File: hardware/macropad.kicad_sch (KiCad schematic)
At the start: 28 parts, among them J1 OLED_128x32, SW1 RotaryEncoder_Switch, U1 Raspberry_Pi_Pico, U2 ESP32-WROOM-32

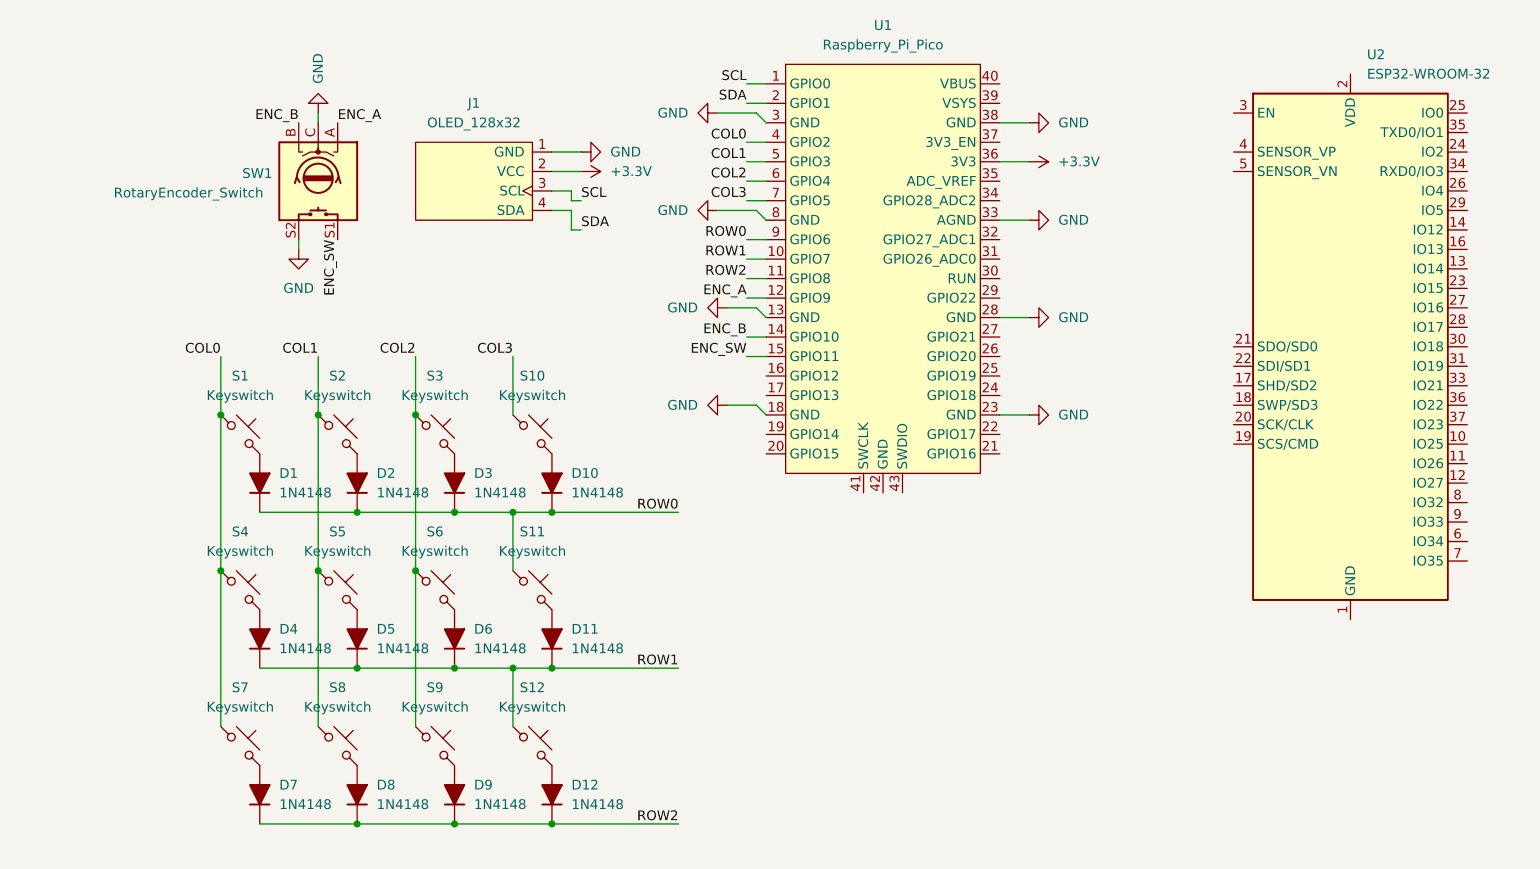
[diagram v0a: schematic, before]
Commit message: updated schematic, removed everything from pcbnew
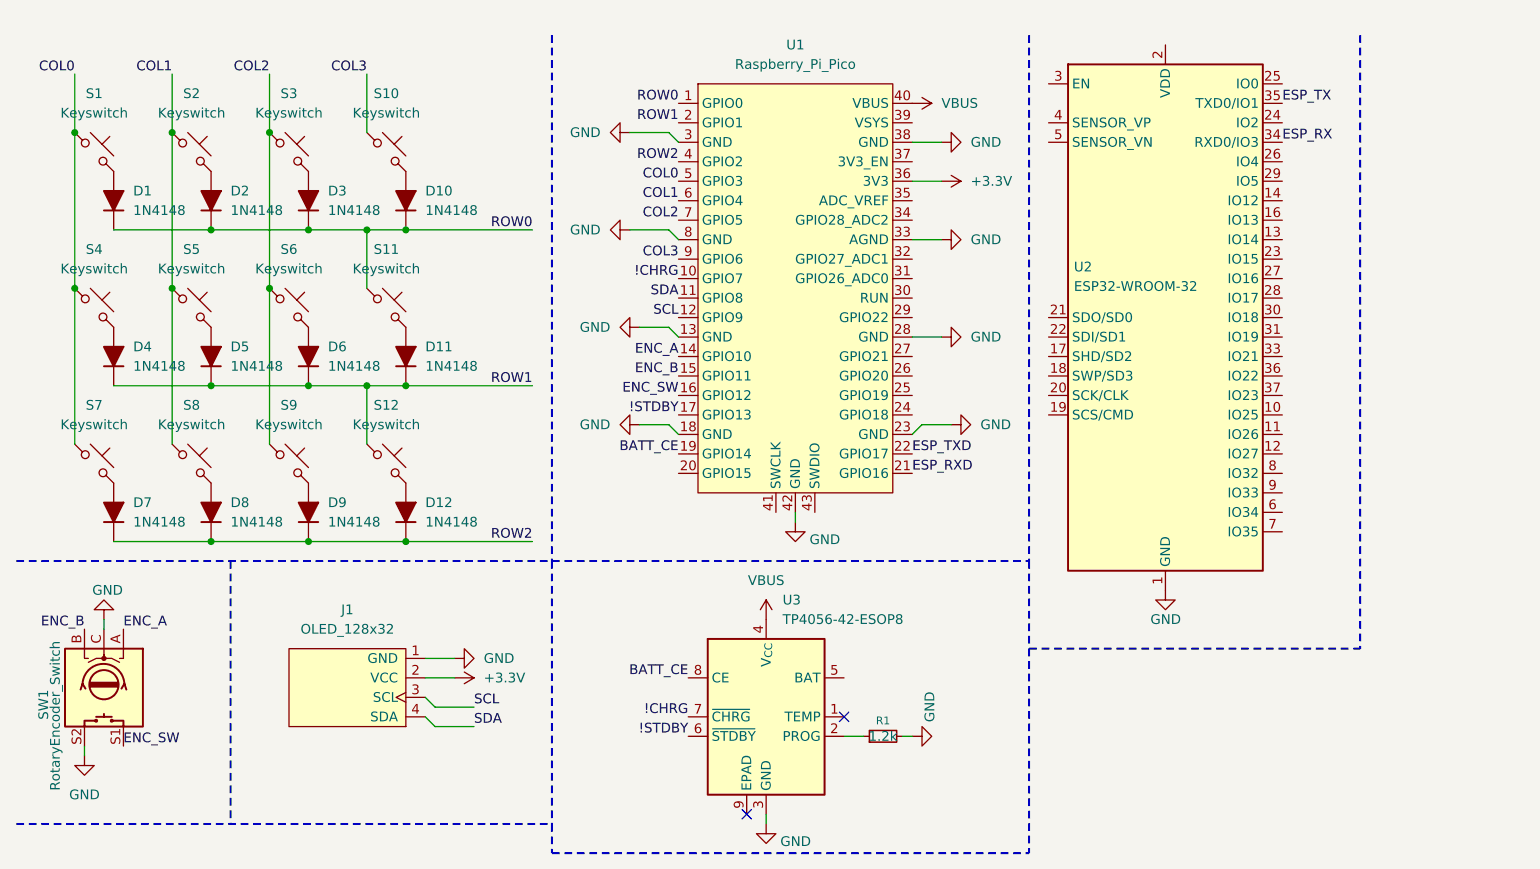
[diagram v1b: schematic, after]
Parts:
- added R1: 1.2k, Resistor_THT:R_Axial_DIN0204_L3.6mm_D1.6mm_P7.62mm_Horizontal, symbol Device:R_Small
- added U3: TP4056-42-ESOP8, Package_SO:SOIC-8-1EP_3.9x4.9mm_P1.27mm_EP2.41x3.3mm_ThermalVias, symbol Battery_Management:TP4056-42-ESOP8
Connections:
- net COL0: now also U1.5 (GPIO3); no longer U1.4 (GPIO2)
- net COL1: now also U1.6 (GPIO4); no longer U1.5 (GPIO3)
- net COL2: now also U1.7 (GPIO5); no longer U1.6 (GPIO4)
- net COL3: now also U1.9 (GPIO6); no longer U1.7 (GPIO5)
- net ENC_A: now also U1.14 (GPIO10); no longer U1.12 (GPIO9)
- net ENC_B: now also U1.15 (GPIO11); no longer U1.14 (GPIO10)
- net ENC_SW: now also U1.16 (GPIO12); no longer U1.15 (GPIO11)
- net GND: now also U1.42 (GND), U2.1 (GND), U2.15 (GND), U2.38 (GND), U2.39 (GND), R1.2, U3.3 (GND)
- net ROW0: now also U1.1 (GPIO0); no longer U1.9 (GPIO6)
- net ROW1: now also U1.2 (GPIO1); no longer U1.10 (GPIO7)
- net ROW2: now also U1.4 (GPIO2); no longer U1.11 (GPIO8)
- net SCL: now also U1.12 (GPIO9); no longer U1.1 (GPIO0)
- net SDA: now also U1.11 (GPIO8); no longer U1.2 (GPIO1)
- net ESP_RX: now reaches U2.34 (RXD0/IO3)
- net ESP_TX: now reaches U2.35 (TXD0/IO1)
- net !STDBY: now reaches U1.17 (GPIO13)
- net !STDBY: now also U3.6 (~{STDBY})
- net BATT_CE: now reaches U1.19 (GPIO14)
- net BATT_CE: now also U3.8 (CE)
- net ESP_RXD: now reaches U1.21 (GPIO16)
- net ESP_TXD: now reaches U1.22 (GPIO17)
- net VBUS: now reaches U1.40 (VBUS)
- net VBUS: now also U3.4 (V_{CC})
- new net: R1.1, U3.2 (PROG)
- new net !CHRG: U1.10 (GPIO7), U3.7 (~{CHRG})
- no-connect marks 0 -> 2
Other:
- moved on the sheet: D1, D10, D11, D12, D2, D3, D4, D5, D6, D7, D8, D9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
